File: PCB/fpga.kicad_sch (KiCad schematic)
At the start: 22 parts, among them IC1 S25FL256LAGMFI003, IC2 LT1932ES6#TRMPBF, J1 0878311420, J4 62684-402100ALF, U4 XC7A100T-FTG256, U5 IS62C1024AL-35QLI-TR, Y2 ECS-3953M-400-BN-TR

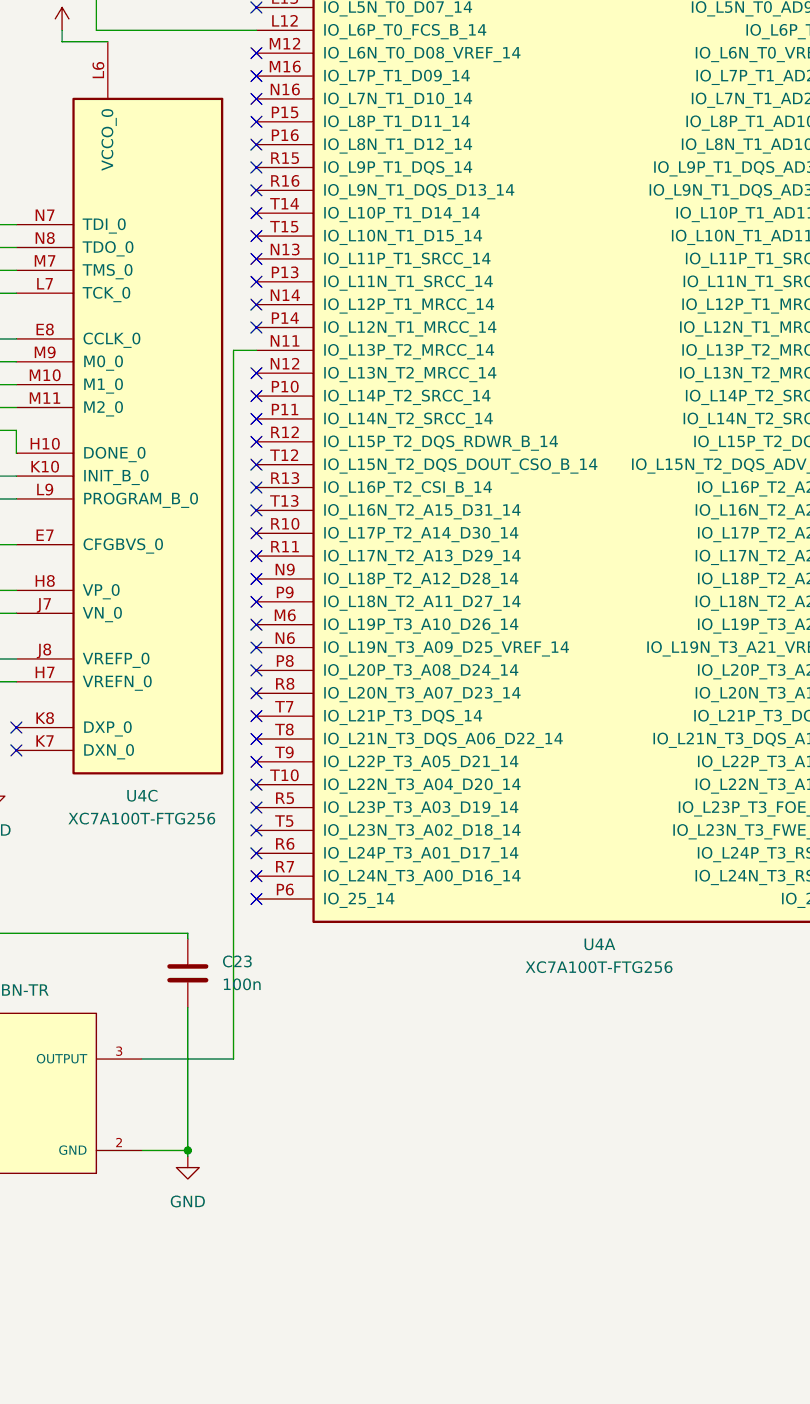
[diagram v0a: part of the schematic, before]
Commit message: updates
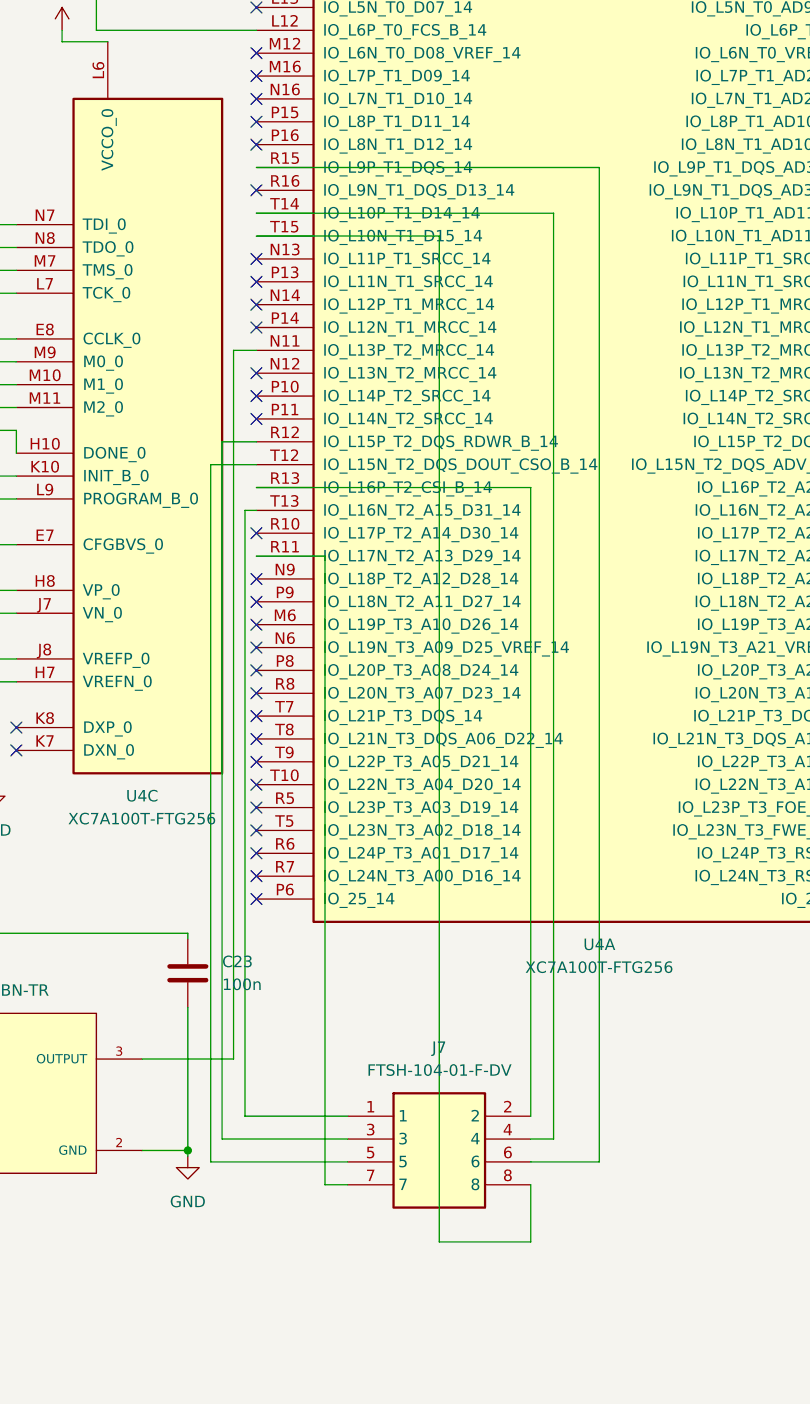
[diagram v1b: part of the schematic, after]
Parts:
- added J7: FTSH-104-01-F-DV, 8pinHeader:FTSH-104-XX-YYY-DV, symbol FTSH-104-01-F-DV:FTSH-104-01-F-DV
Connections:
- net at U4.R11 (IO_L17N_T2_A13_D29_14): now also J7.7
- net at U4.R12 (IO_L15P_T2_DQS_RDWR_B_14): now also J7.3
- net at U4.R13 (IO_L16P_T2_CSI_B_14): now also J7.2
- net at U4.R15 (IO_L9P_T1_DQS_14): now also J7.6
- net at U4.T12 (IO_L15N_T2_DQS_DOUT_CSO_B_14): now also J7.5
- net at U4.T13 (IO_L16N_T2_A15_D31_14): now also J7.1
- net at U4.T14 (IO_L10P_T1_D14_14): now also J7.4
- net at U4.T15 (IO_L10N_T1_D15_14): now also J7.8
- no-connect marks 93 -> 85
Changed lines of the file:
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@@
   (no_connect (at 93.98 148.59))
   (no_connect (at 374.65 134.62))
-  (no_connect (at 93.98 115.57))
   (no_connect (at 381 246.38))
-  (no_connect (at 93.98 118.11))
   (no_connect (at 93.98 72.39))
   (no_connect (at 93.98 156.21))
   (no_connect (at 93.98 110.49))
-  (no_connect (at 93.98 92.71))
   (no_connect (at 167.64 92.71))
   (no_connect (at 93.98 133.35))
@@
   (no_connect (at 374.65 218.44))
   (no_connect (at 167.64 72.39))
-  (no_connect (at 93.98 123.19))
   (no_connect (at 167.64 74.93))
   (no_connect (at 93.98 74.93))
@@
   (no_connect (at 93.98 80.01))
   (no_connect (at 167.64 82.55))
-  (no_connect (at 93.98 120.65))
   (no_connect (at 93.98 77.47))
   (no_connect (at 29.21 50.8))
@@
   (no_connect (at 374.65 129.54))
   (no_connect (at 93.98 158.75))
-  (no_connect (at 93.98 128.27))
   (no_connect (at 93.98 153.67))
   (no_connect (at 29.21 53.34))
@@
   (no_connect (at 93.98 100.33))
   (no_connect (at 381 238.76))
-  (no_connect (at 93.98 90.17))
-  (no_connect (at 93.98 85.09))
   (no_connect (at 93.98 113.03))
   (no_connect (at 374.65 241.3))
@@
     (stroke (width 0) (type default))
   )
+  (wire (pts (xy 114.3 92.71) (xy 93.98 92.71))
+    (stroke (width 0) (type default))
+  )
   (wire (pts (xy 55.88 99.06) (xy 55.88 119.38))
     (stroke (width 0) (type default))
@@
     (stroke (width 0) (type default))
   )
+  (wire (pts (xy 88.9 118.11) (xy 93.98 118.11))
+    (stroke (width 0) (type default))
+  )
   (wire (pts (xy 359.41 87.63) (xy 370.84 87.63))
     (stroke (width 0) (type default))
@@
     (stroke (width 0) (type default))
   )
+  (wire (pts (xy 104.14 198.12) (xy 101.6 198.12))
+    (stroke (width 0) (type default))
+  )
   (wire (pts (xy 167.64 46.99) (xy 171.45 46.99))
     (stroke (width 0) (type default))
@@
     (stroke (width 0) (type default))
   )
+  (wire (pts (xy 101.6 198.12) (xy 101.6 128.27))
+    (stroke (width 0) (type default))
+  )
   (wire (pts (xy 224.79 184.15) (xy 224.79 118.11))
     (stroke (width 0) (type default))
@@
     (stroke (width 0) (type default))
   )
+  (wire (pts (xy 92.71 123.19) (xy 92.71 190.5))
+    (stroke (width 0) (type default))
+  )
   (wire (pts (xy 401.32 95.25) (xy 370.84 95.25))
     (stroke (width 0) (type default))
@@
     (stroke (width 0) (type default))
   )
+  (wire (pts (xy 93.98 128.27) (xy 101.6 128.27))
+    (stroke (width 0) (type default))
+  )
   (wire (pts (xy 208.28 161.29) (xy 214.63 161.29))
     (stroke (width 0) (type default))
@@
     (stroke (width 0) (type default))
   )
+  (wire (pts (xy 104.14 193.04) (xy 90.17 193.04))
+    (stroke (width 0) (type default))
+  )
+  (wire (pts (xy 88.9 195.58) (xy 88.9 118.11))
+    (stroke (width 0) (type default))
+  )
   (wire (pts (xy 273.05 72.39) (xy 273.05 74.93))
     (stroke (width 0) (type default))
   )
+  (wire (pts (xy 93.98 85.09) (xy 132.08 85.09))
+    (stroke (width 0) (type default))
+  )
   (wire (pts (xy 15.24 114.3) (xy 16.51 114.3))
     (stroke (width 0) (type default))
@@
     (stroke (width 0) (type default))
   )
+  (wire (pts (xy 124.46 195.58) (xy 132.08 195.58))
+    (stroke (width 0) (type default))
+  )
   (wire (pts (xy 60.96 93.98) (xy 67.31 93.98))
     (stroke (width 0) (type default))
@@
     (stroke (width 0) (type default))
   )
+  (wire (pts (xy 132.08 85.09) (xy 132.08 195.58))
+    (stroke (width 0) (type default))
+  )
   (wire (pts (xy 262.89 137.16) (xy 273.05 137.16))
     (stroke (width 0) (type default))
@@
     (stroke (width 0) (type default))
   )
+  (wire (pts (xy 93.98 90.17) (xy 127 90.17))
+    (stroke (width 0) (type default))
+  )
   (wire (pts (xy 168.91 130.81) (xy 168.91 129.54))
     (stroke (width 0) (type default))
@@
     (stroke (width 0) (type default))
   )
+  (wire (pts (xy 104.14 195.58) (xy 88.9 195.58))
+    (stroke (width 0) (type default))
+  )
   (wire (pts (xy 82.55 33.02) (xy 82.55 48.26))
     (stroke (width 0) (type default))
@@
     (stroke (width 0) (type default))
   )
+  (wire (pts (xy 93.98 123.19) (xy 92.71 123.19))
+    (stroke (width 0) (type default))
+  )
   (wire (pts (xy 406.4 147.32) (xy 406.4 149.86))
     (stroke (width 0) (type default))
@@
     (stroke (width 0) (type default))
   )
+  (wire (pts (xy 124.46 204.47) (xy 124.46 198.12))
+    (stroke (width 0) (type default))
+  )
   (wire (pts (xy 240.03 85.09) (xy 240.03 87.63))
     (stroke (width 0) (type default))
@@
     (stroke (width 0) (type default))
   )
+  (wire (pts (xy 114.3 92.71) (xy 114.3 204.47))
+    (stroke (width 0) (type default))
+  )
   (wire (pts (xy 63.5 91.44) (xy 67.31 91.44))
     (stroke (width 0) (type default))
@@
     (stroke (width 0) (type default))
   )
+  (wire (pts (xy 104.14 190.5) (xy 92.71 190.5))
+    (stroke (width 0) (type default))
+  )
   (wire (pts (xy 50.8 104.14) (xy 67.31 104.14))
     (stroke (width 0) (type default))
@@
     (stroke (width 0) (type default))
   )
+  (wire (pts (xy 90.17 115.57) (xy 93.98 115.57))
+    (stroke (width 0) (type default))
+  )
   (wire (pts (xy 50.8 104.14) (xy 50.8 67.31))
     (stroke (width 0) (type default))
@@
     (stroke (width 0) (type default))
   )
+  (wire (pts (xy 124.46 190.5) (xy 124.46 120.65))
+    (stroke (width 0) (type default))
+  )
   (wire (pts (xy 168.91 129.54) (xy 218.44 129.54))
     (stroke (width 0) (type default))
@@
     (stroke (width 0) (type default))
   )
+  (wire (pts (xy 127 90.17) (xy 127 193.04))
+    (stroke (width 0) (type default))
+  )
   (wire (pts (xy 29.21 60.96) (xy 29.21 67.31))
     (stroke (width 0) (type default))
@@
     (stroke (width 0) (type default))
   )
+  (wire (pts (xy 124.46 193.04) (xy 127 193.04))
+    (stroke (width 0) (type default))
+  )
   (wire (pts (xy 15.24 127) (xy 15.24 124.46))
     (stroke (width 0) (type default))
@@
     (stroke (width 0) (type default))
   )
+  (wire (pts (xy 124.46 120.65) (xy 93.98 120.65))
+    (stroke (width 0) (type default))
+  )
   (wire (pts (xy 240.03 62.23) (xy 240.03 64.77))
     (stroke (width 0) (type default))
@@
     (stroke (width 0) (type default))
   )
+  (wire (pts (xy 90.17 115.57) (xy 90.17 193.04))
+    (stroke (width 0) (type default))
+  )
   (wire (pts (xy 50.8 105.41) (xy 54.61 105.41))
     (stroke (width 0) (type default))
@@
     (stroke (width 0) (type default))
   )
+  (wire (pts (xy 114.3 204.47) (xy 124.46 204.47))
+    (stroke (width 0) (type default))
+  )
   (wire (pts (xy 240.03 41.91) (xy 240.03 43.18))
     (stroke (width 0) (type default))
@@
         )
       )
+    )
+  )
+  (symbol (lib_id "FTSH-104-01-F-DV:FTSH-104-01-F-DV") (at 104.14 190.5 0) (unit 1)
+    (in_bom yes) (on_board yes) (dnp no) (fields_autoplaced)
+    (property "Reference" "J7" (at 114.3 182.88 0)
+      (effects (font (size 1.27 1.27)))
+    )
+    (property "Value" "FTSH-104-01-F-DV" (at 114.3 185.42 0)
+      (effects (font (size 1.27 1.27)))
+    )
+    (property "Footprint" "8pinHeader:FTSH-104-XX-YYY-DV" (at 120.65 285.42 0)
+      (effects (font (size 1.27 1.27)) (justify left top) hide)
+    )
+    (property "Datasheet" "http://suddendocs.samtec.com/prints/ftsh-1xx-xx-xxx-dv-xxx-xxx-mkt.pdf" (at 120.65 385.42 0)
+      (effects (font (size 1.27 1.27)) (justify left top) hide)
+    )
+    (property "Height" "" (at 120.65 585.42 0)
+      (effects (font (size 1.27 1.27)) (justify left top) hide)
+    )
+    (property "Manufacturer_Name" "SAMTEC" (at 120.65 685.42 0)
+      (effects (font (size 1.27 1.27)) (justify left top) hide)
+    )
+    (property "Manufacturer_Part_Number" "FTSH-104-01-F-DV" (at 120.65 785.42 0)
+      (effects (font (size 1.27 1.27)) (justify left top) hide)
+    )
+    (property "Mouser Part Number" "200-FTSH10401FDV" (at 120.65 885.42 0)
+      (effects (font (size 1.27 1.27)) (justify left top) hide)
+    )
+    (property "Mouser Price/Stock" "https://www.mouser.co.uk/ProductDetail/Samtec/FTSH-104-01-F-DV?qs=0lQeLiL1qyausn2wOF0W5g%3D%3D" (at 120.65 985.42 0)
+      (effects (font (size 1.27 1.27)) (justify left top) hide)
+    )
+    (property "Arrow Part Number" "FTSH-104-01-F-DV" (at 120.65 1085.42 0)
+      (effects (font (size 1.27 1.27)) (justify left top) hide)
+    )
+    (property "Arrow Price/Stock" "https://www.arrow.com/en/products/ftsh-104-01-f-dv/samtec?region=nac" (at 120.65 1185.42 0)
+      (effects (font (size 1.27 1.27)) (justify left top) hide)
+    )
+    (pin "1")
+    (pin "2")
+    (pin "3")
+    (pin "4")
+    (pin "5")
+    (pin "6")
+    (pin "7")
+    (pin "8")
+    (instances
+      (project "PCB"
+        (path "/aa113cd6-c3ac-4890-9a84-1ea195994408/e43e14ef-0971-4dbf-9758-48ad88cea06a"
+          (reference "J7") (unit 1)
+        )
+      )
